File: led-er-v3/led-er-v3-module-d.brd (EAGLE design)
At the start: 157 x 59 mm, 41 parts

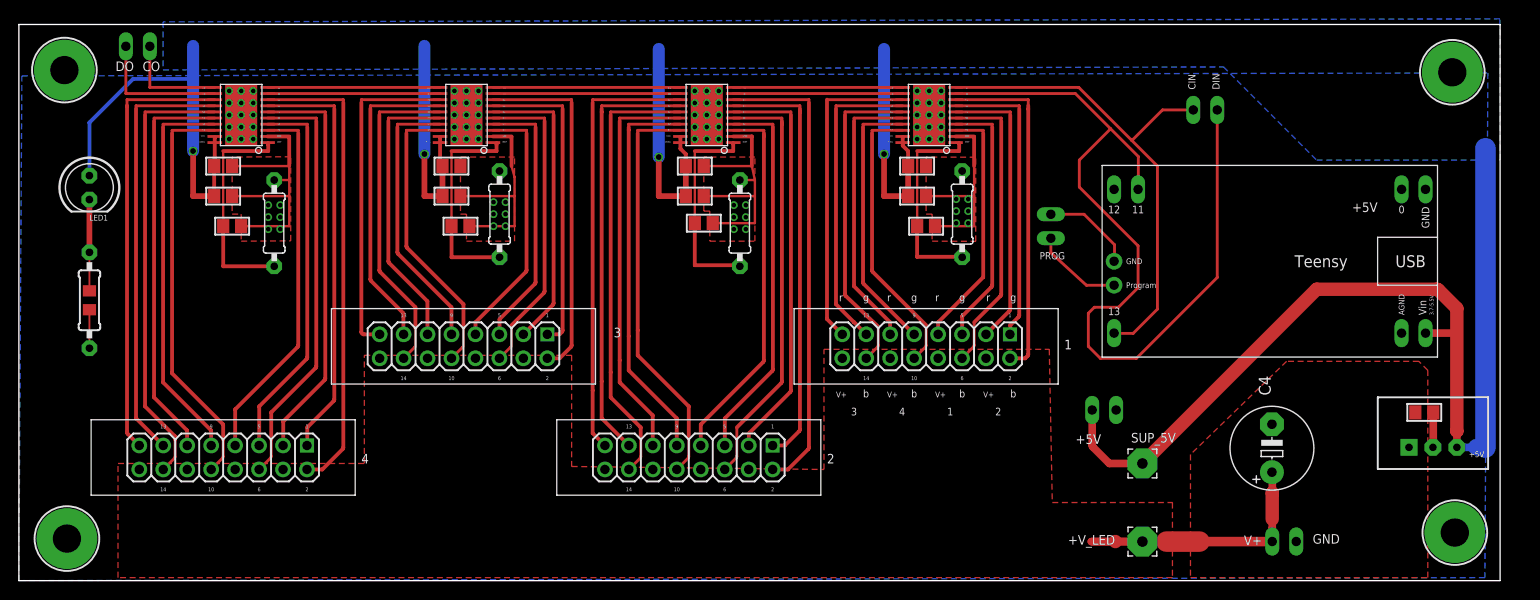
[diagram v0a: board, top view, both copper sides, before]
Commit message: long and skinny working
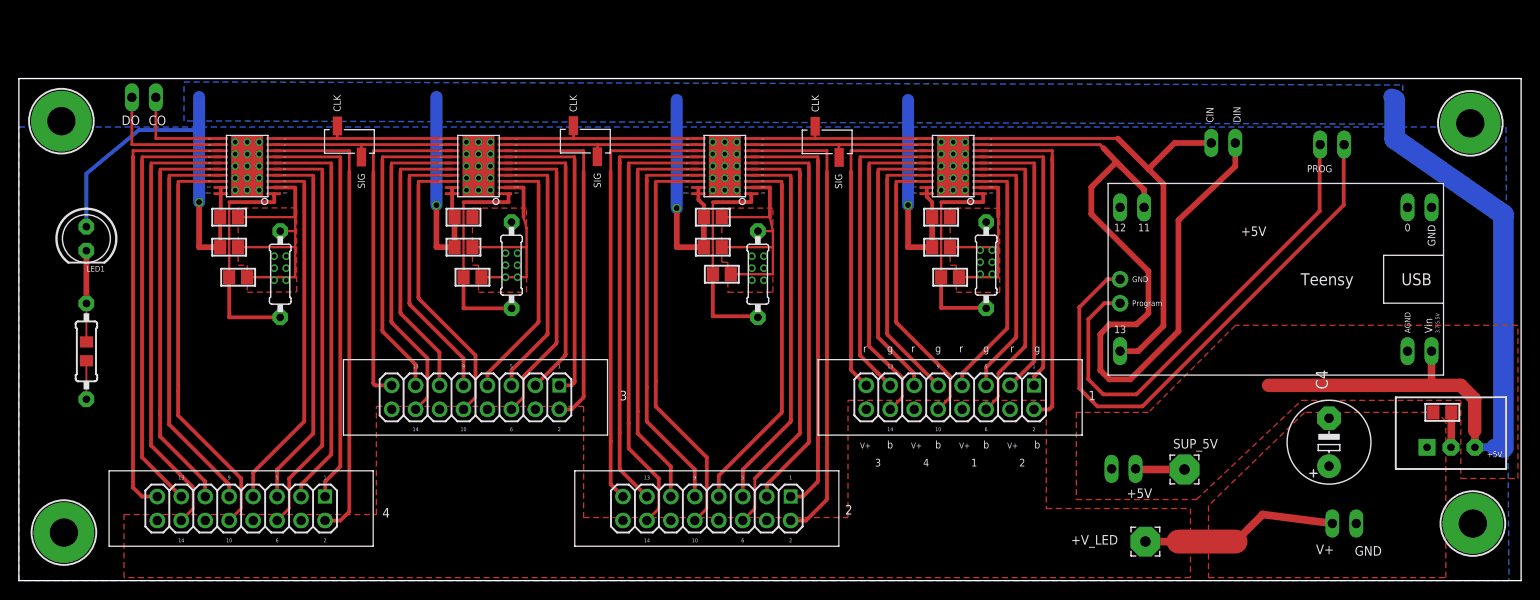
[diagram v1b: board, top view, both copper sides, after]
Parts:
- added JP1, JP2, JP3: (no value), Andrews:1X06_SMD_STRAIGHT_ALT
- moved JP_PROG 31.1 mm to (139.2, 46.2), turned to 180 degrees
- moved JP_15VIN 6.65 mm to (140.5, 6.06)
- moved JP_5V 6.58 mm to (117.1, 11.8), turned to 0 degrees
- moved C4 6.09 mm to (138.9, 14.7)
- moved LED-ER1:C11 5.98 mm to (97.8, 35.4)
- moved LED-ER1:C5 5.98 mm to (97.8, 38.5)
- moved LED-ER1:R6 5.98 mm to (102.6, 33.4)
- moved LED-ER1:TLC1 5.98 mm to (99.1, 44.0)
- moved LED-ER1:U$6 5.98 mm to (98.7, 19.4)
- moved LED-ER1:R3 5.98 mm to (98.7, 32.2)
- moved LED-ER2:R3 5.74 mm to (74.5, 32.5)
- moved LED-ER2:R6 5.74 mm to (78.4, 32.5)
- moved LED-ER2:U$6 5.74 mm to (72.9, 7.64)
- moved LED-ER4:U$6 5.74 mm to (23.6, 7.64)
- moved LED-ER2:C11 5.74 mm to (73.6, 35.4)
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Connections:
- net N$2: now also JP1.2
- net N$3: now also JP1.1
- net N$4: now also JP2.2
- net N$5: now also JP2.1
- net N$6: now also JP3.2
- net N$7: now also JP3.1
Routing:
- net N$54: track 9.86 -> 58.2 mm
- net N$55: track 9.58 -> 50.8 mm
- net +5V: track 232.6 -> 201.2 mm
- net VIN: track 32.0 -> 21.1 mm
- net 1SDTI: track 91.9 -> 84.8 mm
- net 1SCKI: track 53.6 -> 50.1 mm
- net N$3: track 18.0 -> 20.0 mm
- net N$5: track 19.9 -> 21.9 mm
- net N$4: track 19.9 -> 21.9 mm
- net N$6: track 18.3 -> 20.3 mm
- net N$7: track 18.3 -> 20.2 mm
- net N$2: track 18.0 -> 19.9 mm
- net LED-ER4:R2: track 46.5 -> 48.0 mm
- net LED-ER4:B3: track 43.2 -> 43.8 mm
- net LED-ER4:B2: track 47.1 -> 47.7 mm
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- added copper zone on layer 1, net +5V
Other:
- board size 157 x 59 mm -> 159.3 x 53.2 mm
- board text added: "CLK"
- board text added: "SIG"
